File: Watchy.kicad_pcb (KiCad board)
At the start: 2 copper layers, 33.8 x 46 mm, 70 parts, among them J1 FPC24(0.5MM), J2 Micro USB, J3 Battery, M1 Vibration_Motor, Q1 AO3400A, Q2 UMH3N, Q4 CJ2301, Q5 S8050, SW1 BTN, SW2 BTN, SW3 BTN, SW4 BTN, U1 ESP32-PICO-D4, U2 ME6211C33M5G-N, U3 CP2102, U4 BMA423, U5 TP4054, U6 PCF8563BS, Y1 32.768KHz

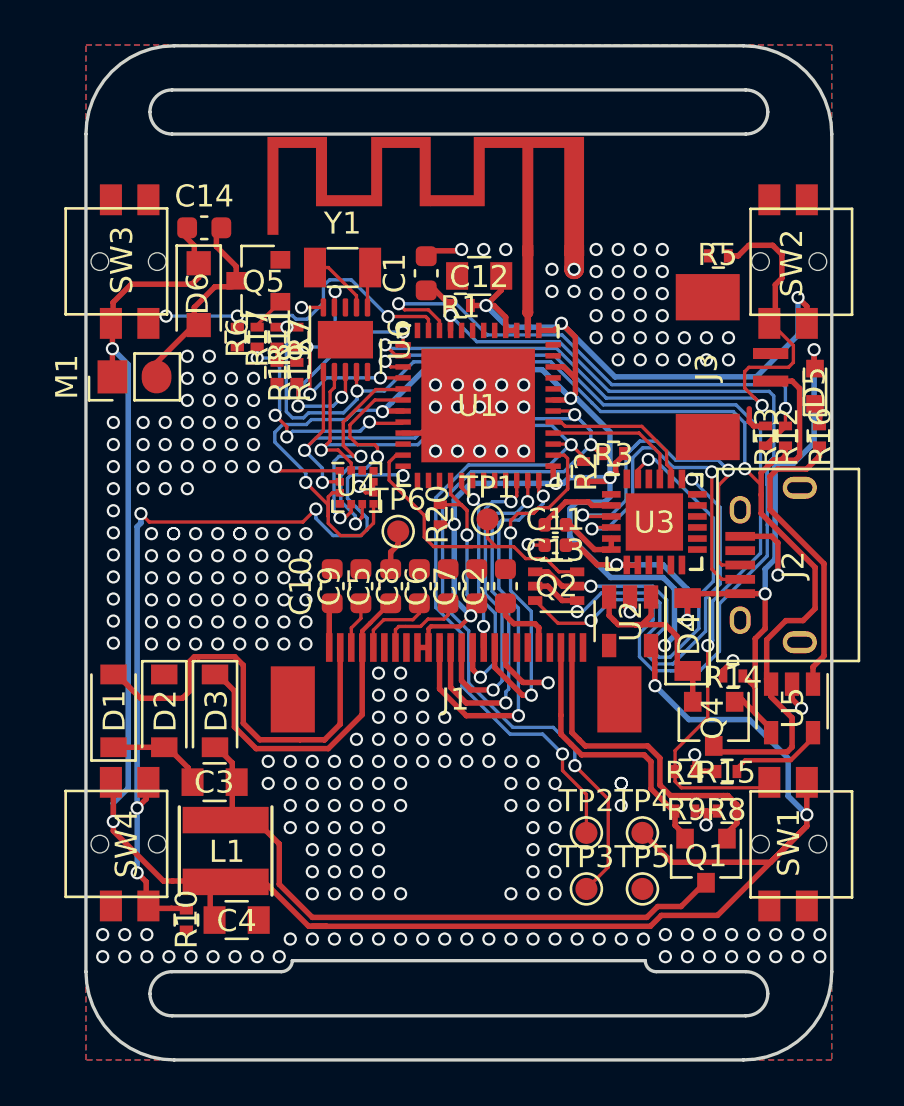
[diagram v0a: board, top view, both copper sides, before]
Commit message: update to kicad 7
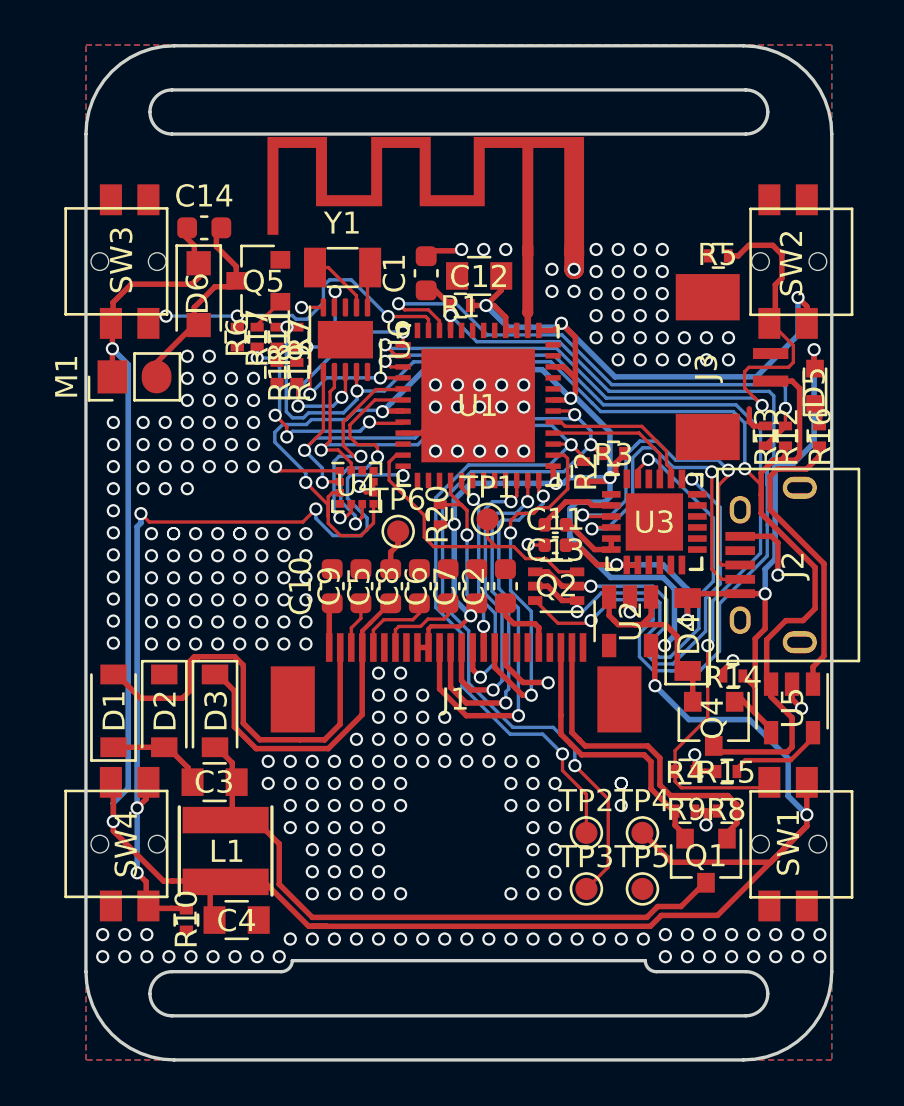
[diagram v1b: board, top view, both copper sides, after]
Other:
- net class Default removed
